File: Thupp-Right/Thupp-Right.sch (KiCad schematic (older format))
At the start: 43 parts, among them U1 nice_nano

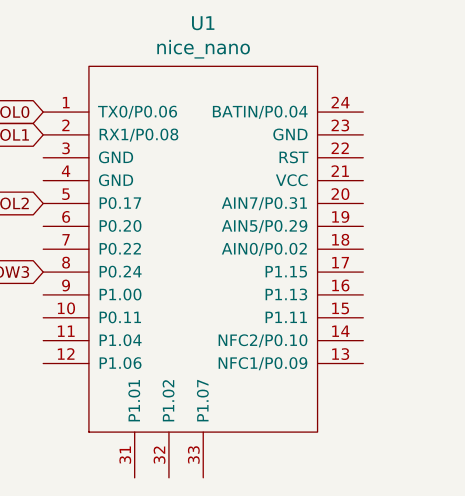
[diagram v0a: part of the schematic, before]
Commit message: fully routed 1st attempt
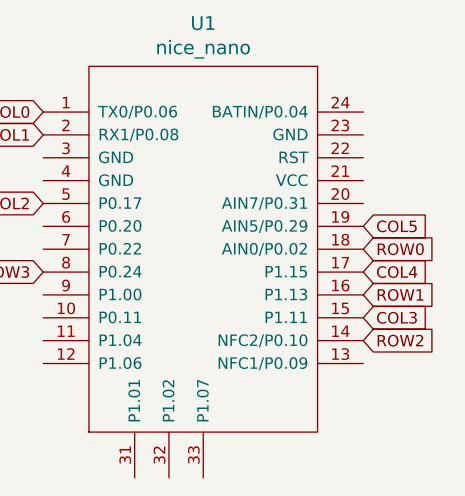
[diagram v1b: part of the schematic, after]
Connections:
- net COL3: now also U1.15 (P1.11)
- net COL4: now also U1.17 (P1.15)
- net COL5: now also U1.19 (AIN5/P0.29)
- net ROW0: now also U1.18 (AIN0/P0.02)
- net ROW1: now also U1.16 (P1.13)
- net ROW2: now also U1.14 (NFC2/P0.10)
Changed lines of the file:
@@
 	1300 1450 1200 1450
-$Comp
-L Device:D_Small D1
-U 1 1 6179D221
-P 1200 1550
-F 0 "D1" V 1246 1480 50  0000 R CNN
-F 1 "D_Small" V 1155 1480 50  0000 R CNN
-F 2 "Diode_SMD:D_SOD-123" V 1200 1550 50  0001 C CNN
-F 3 "~" V 1200 1550 50  0001 C CNN
-	1    1200 1550
-	0    -1   -1   0
-$EndComp
 $Comp
 L MX_Alps_Hybrid:MX-NoLED MX2
@@
 Text GLabel 3000 3900 0    50   Input ~ 0
 COL0
+$Comp
+L Device:D_Small D1
+U 1 1 6179D221
+P 1200 1550
+F 0 "D1" V 1246 1480 50  0000 R CNN
+F 1 "D_Small" V 1155 1480 50  0000 R CNN
+F 2 "Diode_SMD:D_SOD-123" V 1200 1550 50  0001 C CNN
+F 3 "~" V 1200 1550 50  0001 C CNN
+	1    1200 1550
+	0    -1   -1   0
+$EndComp
+Text GLabel 4400 4900 2    50   Input ~ 0
+ROW2
+Text GLabel 4400 4800 2    50   Input ~ 0
+COL3
+Text GLabel 4400 4700 2    50   Input ~ 0
+ROW1
+Text GLabel 4400 4600 2    50   Input ~ 0
+COL4
+Text GLabel 4400 4500 2    50   Input ~ 0
+ROW0
+Text GLabel 4400 4400 2    50   Input ~ 0
+COL5
 $EndSCHEMATC
